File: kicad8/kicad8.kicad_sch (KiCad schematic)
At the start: 21 parts, among them J1 USB_C_Receptacle_USB2.0, U1 STM32F072CBT6, U2 PRTR5V0U2X

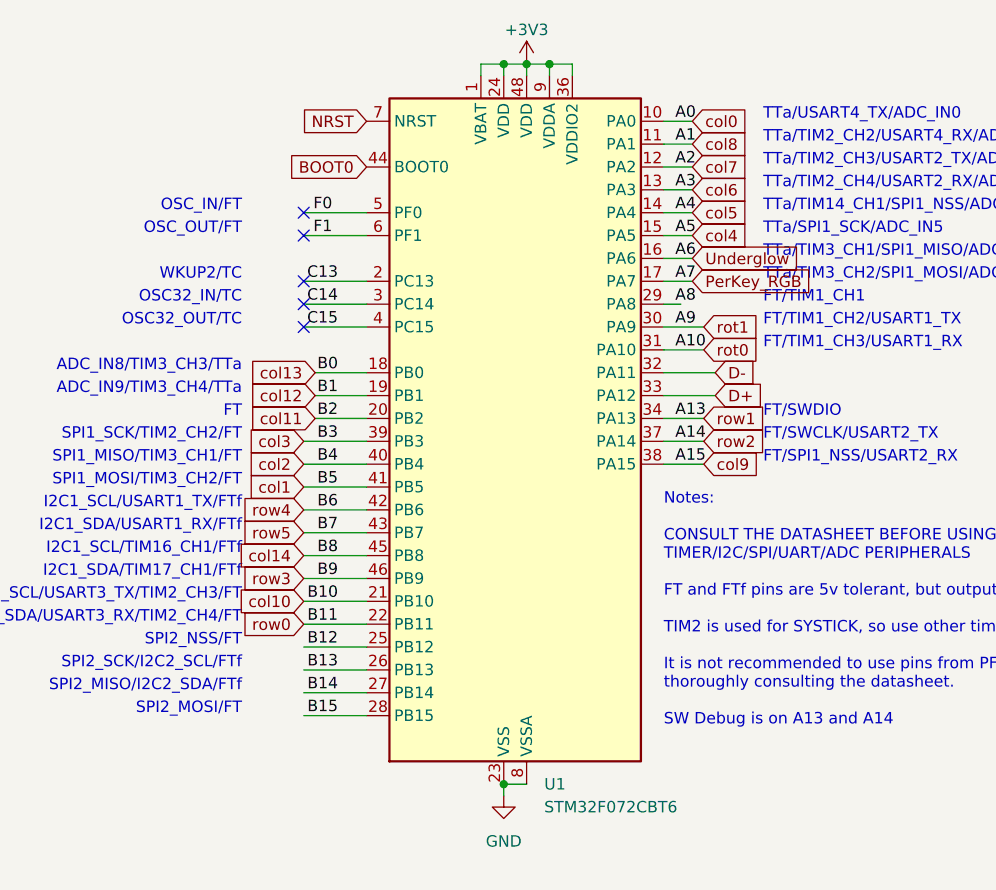
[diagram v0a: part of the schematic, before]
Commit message: Initial branch commit
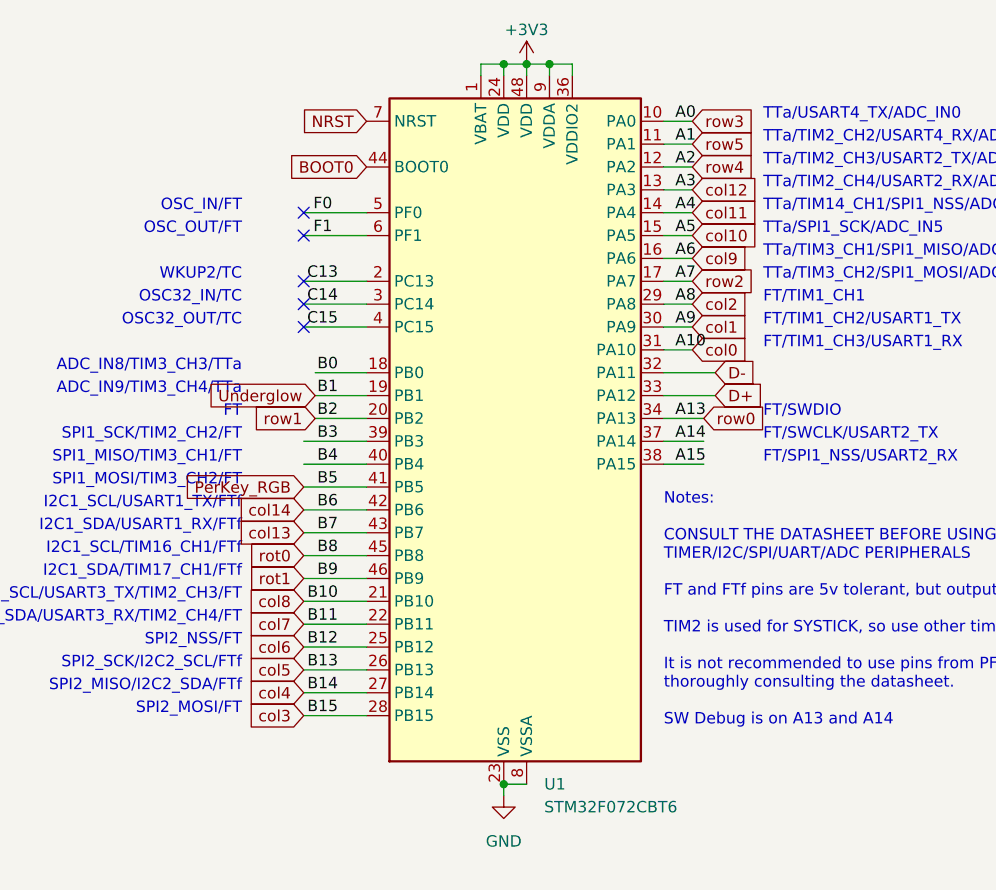
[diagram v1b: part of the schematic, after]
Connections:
- net A8 is gone; now on net col2: U1.29 (PA8)
- net B12 is gone; now on net col6: U1.25 (PB12)
- net B13 is gone; now on net col5: U1.26 (PB13)
- net B14 is gone; now on net col4: U1.27 (PB14)
- net B15 is gone; now on net col3: U1.28 (PB15)
- net PerKey_RGB: now also U1.41 (PB5); no longer U1.17 (PA7)
- net Underglow: now also U1.19 (PB1); no longer U1.16 (PA6)
- net col0: now also U1.31 (PA10); no longer U1.10 (PA0)
- net col1: now also U1.30 (PA9); no longer U1.41 (PB5)
- net col10: now also U1.15 (PA5); no longer U1.21 (PB10)
- net col11: now also U1.14 (PA4); no longer U1.20 (PB2)
- net col12: now also U1.13 (PA3); no longer U1.19 (PB1)
- net col13: now also U1.43 (PB7); no longer U1.18 (PB0)
- net col14: now also U1.42 (PB6); no longer U1.45 (PB8)
- net col2: no longer U1.40 (PB4)
- net col3: no longer U1.39 (PB3)
- net col4: no longer U1.15 (PA5)
- net col5: no longer U1.14 (PA4)
- net col6: no longer U1.13 (PA3)
- net col7: now also U1.22 (PB11); no longer U1.12 (PA2)
- net col8: now also U1.21 (PB10); no longer U1.11 (PA1)
- net col9: now also U1.16 (PA6); no longer U1.38 (PA15)
- net rot0: now also U1.45 (PB8); no longer U1.31 (PA10)
- net rot1: now also U1.46 (PB9); no longer U1.30 (PA9)
- net row0: now also U1.34 (PA13); no longer U1.22 (PB11)
- net row1: now also U1.20 (PB2); no longer U1.34 (PA13)
- net row2: now also U1.17 (PA7); no longer U1.37 (PA14)
- net row3: now also U1.10 (PA0); no longer U1.46 (PB9)
- net row4: now also U1.12 (PA2); no longer U1.42 (PB6)
- net row5: now also U1.11 (PA1); no longer U1.43 (PB7)
- new net A14: U1.37 (PA14)
- new net A15: U1.38 (PA15)
- new net B0: U1.18 (PB0)
- new net B3: U1.39 (PB3)
- new net B4: U1.40 (PB4)
